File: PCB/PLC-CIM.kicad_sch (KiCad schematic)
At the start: 3 parts, among them IC31 TXS0102DCUTG4, U1 ESP32-DEVKITC

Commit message: Revert "Revert "# Title: Summary, imperative, start upper case, don't end with a period""
This reverts commit 3a20dd9da141c7cb1bae8077342d3450242b15f5.
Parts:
- IC31: footprint SOP50P310X90-8N -> TXS0102DCUTG4:SOP50P310X90-8N
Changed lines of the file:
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@@
       (effects (font (size 1.27 1.27)))
     )
-    (property "Footprint" "SOP50P310X90-8N" (at 222.25 237.795 0)
+    (property "Footprint" "TXS0102DCUTG4:SOP50P310X90-8N" (at 222.25 237.795 0)
       (effects (font (size 1.27 1.27)) (justify left top) hide)
     )

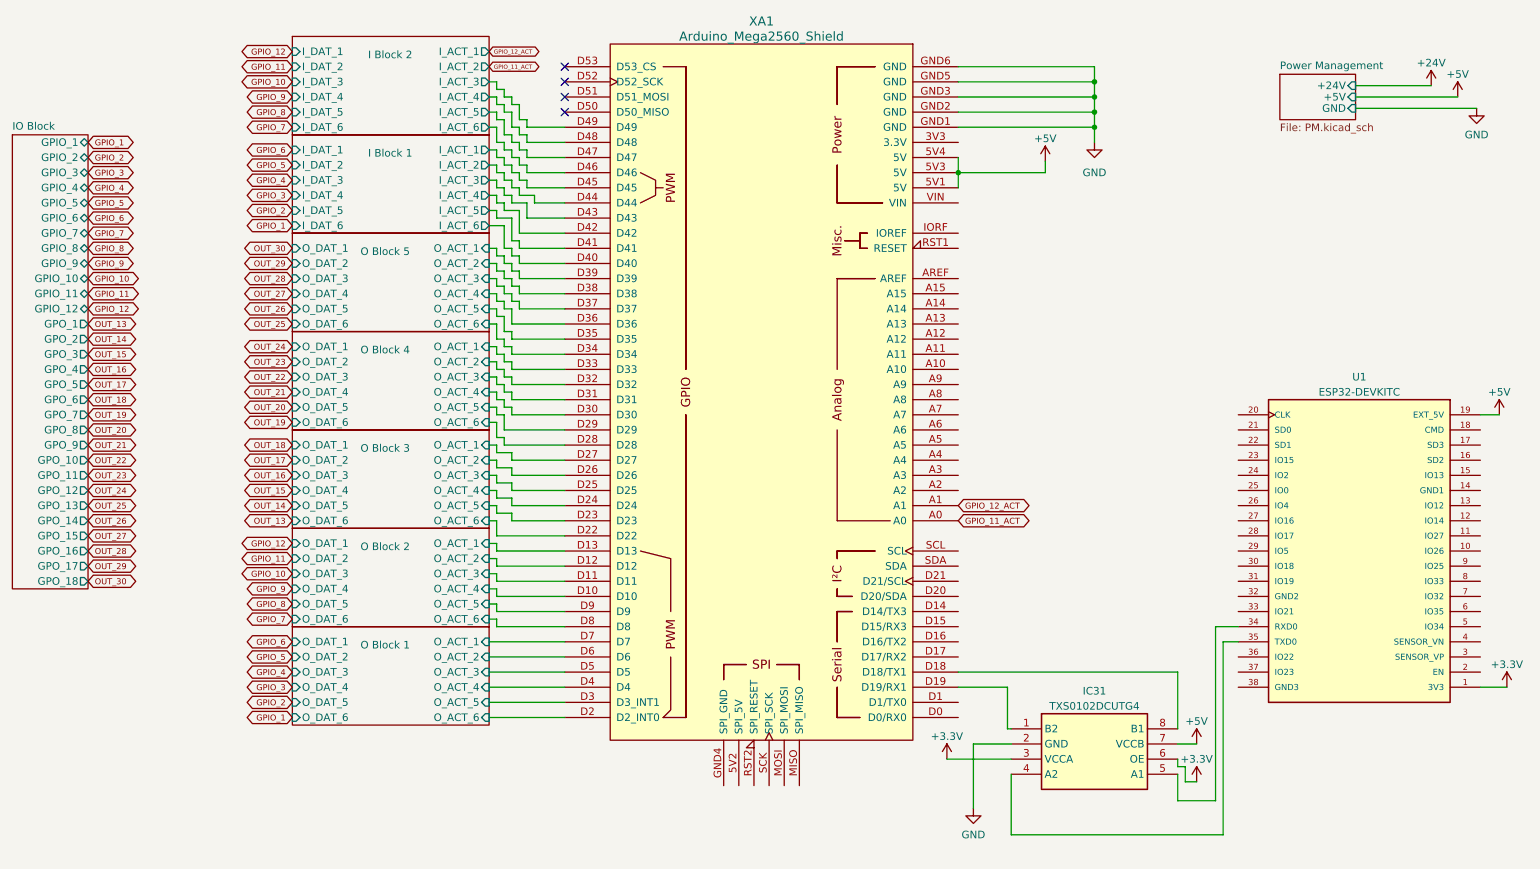
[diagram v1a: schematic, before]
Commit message: Finalized generalized design
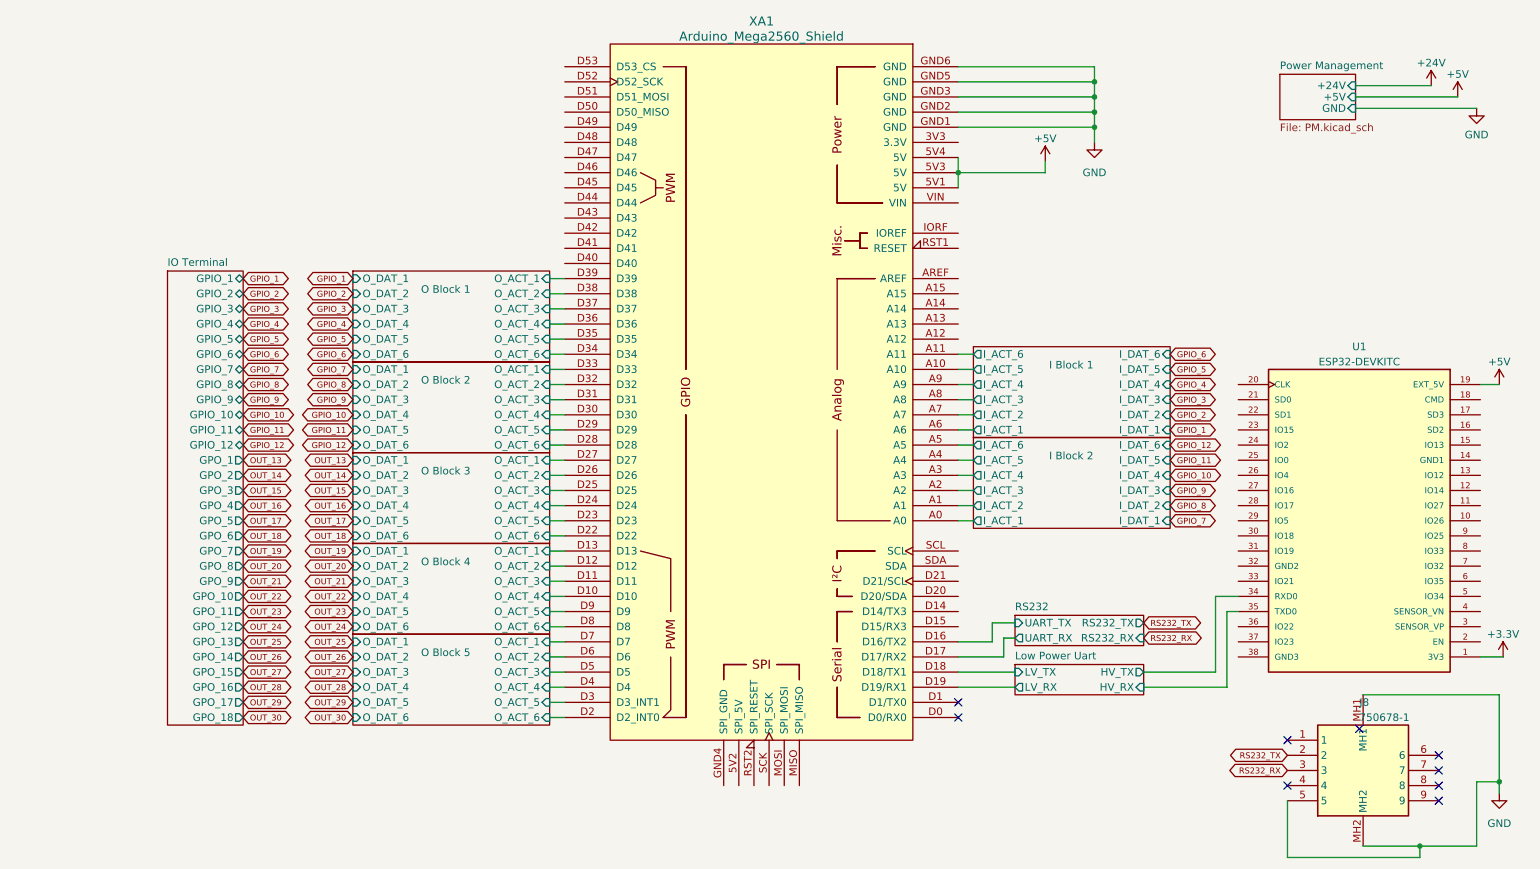
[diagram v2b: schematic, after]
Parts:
- removed IC31: TXS0102DCUTG4, TXS0102DCUTG4:SOP50P310X90-8N, symbol TXS0102DCUTG4:TXS0102DCUTG4
- added J8: 750678-1, 7506781, symbol 750678-1:750678-1
- U1: MANUFACTURER ESPRESSIF -> (none); Manufacturer_Name (none) -> Espressif; Manufacturer_Part_Number (none) -> ESP32-DevKitC V4; Mouser Part Number (none) -> 356-ESP32-DEVKITC; Mouser Price/Stock (none) -> https://eu.mouser.com/ProductDetail/Espressif-Systems/ESP32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
- XA1: Manufacturer_Name (none) -> DFRobot; Manufacturer_Part_Number (none) -> DFR0108; Mouser Part Number (none) -> 426-DFR0108; Mouser Price/Stock (none) -> https://eu.mouser.com/ProductDetail/DFRobot/DFR0108?qs=5aG0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
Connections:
- net GND: now also J8.5, J8.MH1, J8.MH2
- net I Block 1/I_ACT_1: now also XA1.A6; no longer XA1.D45
- net I Block 1/I_ACT_2: now also XA1.A7; no longer XA1.D44
- net I Block 1/I_ACT_3: now also XA1.A8; no longer XA1.D43
- net I Block 1/I_ACT_4: now also XA1.A9; no longer XA1.D42
- net I Block 1/I_ACT_5: now also XA1.A10; no longer XA1.D41
- net I Block 1/I_ACT_6: now also XA1.A11; no longer XA1.D40
- net I Block 2/I_ACT_3: now also XA1.A2; no longer XA1.D49
- net I Block 2/I_ACT_4: now also XA1.A3; no longer XA1.D48
- net I Block 2/I_ACT_5: now also XA1.A4; no longer XA1.D47
- net I Block 2/I_ACT_6: now also XA1.A5; no longer XA1.D46
- net O Block 1/O_ACT_1: now also XA1.D39; no longer XA1.D7
- net O Block 1/O_ACT_2: now also XA1.D38; no longer XA1.D6
- net O Block 1/O_ACT_3: now also XA1.D37; no longer XA1.D5
- net O Block 1/O_ACT_4: now also XA1.D36; no longer XA1.D4
- net O Block 1/O_ACT_5: now also XA1.D35; no longer XA1.D3 (D3_INT1)
- net O Block 1/O_ACT_6: now also XA1.D34; no longer XA1.D2 (D2_INT0)
- net O Block 2/O_ACT_1: now also XA1.D33; no longer XA1.D13
- net O Block 2/O_ACT_2: now also XA1.D32; no longer XA1.D12
- net O Block 2/O_ACT_3: now also XA1.D31; no longer XA1.D11
- net O Block 2/O_ACT_4: now also XA1.D30; no longer XA1.D10
- net O Block 2/O_ACT_5: now also XA1.D29; no longer XA1.D9
- net O Block 2/O_ACT_6: now also XA1.D28; no longer XA1.D8
- net O Block 4/O_ACT_1: now also XA1.D13; no longer XA1.D33
- net O Block 4/O_ACT_2: now also XA1.D12; no longer XA1.D32
- net O Block 4/O_ACT_3: now also XA1.D11; no longer XA1.D31
- net O Block 4/O_ACT_4: now also XA1.D10; no longer XA1.D30
- net O Block 4/O_ACT_5: now also XA1.D9; no longer XA1.D29
- net O Block 4/O_ACT_6: now also XA1.D8; no longer XA1.D28
- net O Block 5/O_ACT_1: now also XA1.D7; no longer XA1.D39
- net O Block 5/O_ACT_2: now also XA1.D6; no longer XA1.D38
- net O Block 5/O_ACT_3: now also XA1.D5; no longer XA1.D37
- net O Block 5/O_ACT_4: now also XA1.D4; no longer XA1.D36
- net O Block 5/O_ACT_5: now also XA1.D3 (D3_INT1); no longer XA1.D35
- net O Block 5/O_ACT_6: now also XA1.D2 (D2_INT0); no longer XA1.D34
- net Low Power Uart/LV_RX: now reaches XA1.D19 (D19/RX1)
- net Low Power Uart/HV_RX: now reaches U1.35 (TXD0)
- net Low Power Uart/HV_TX: now reaches U1.34 (RXD0)
- net Low Power Uart/LV_TX: now reaches XA1.D18 (D18/TX1)
- net RS232/UART_TX: now reaches XA1.D16 (D16/TX2)
- net RS232/UART_RX: now reaches XA1.D17 (D17/RX2)
- net GPIO_11_ACT renamed I Block 2/I_ACT_1
- net GPIO_12_ACT renamed I Block 2/I_ACT_2
- new net RS232_RX: J8.3
- new net RS232_TX: J8.2
- no-connect marks 4 -> 9
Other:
- sheet IO Block renamed IO Terminal
- added sheet Low Power Uart (lp_uart_block.kicad_sch)
- added sheet RS232 (RS232.kicad_sch)
- moved on the sheet: U1
